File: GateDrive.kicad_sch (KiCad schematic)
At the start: 31 parts, among them Q4 BSS123, U1 UCC21330BQDRQ1, U4 IR2184

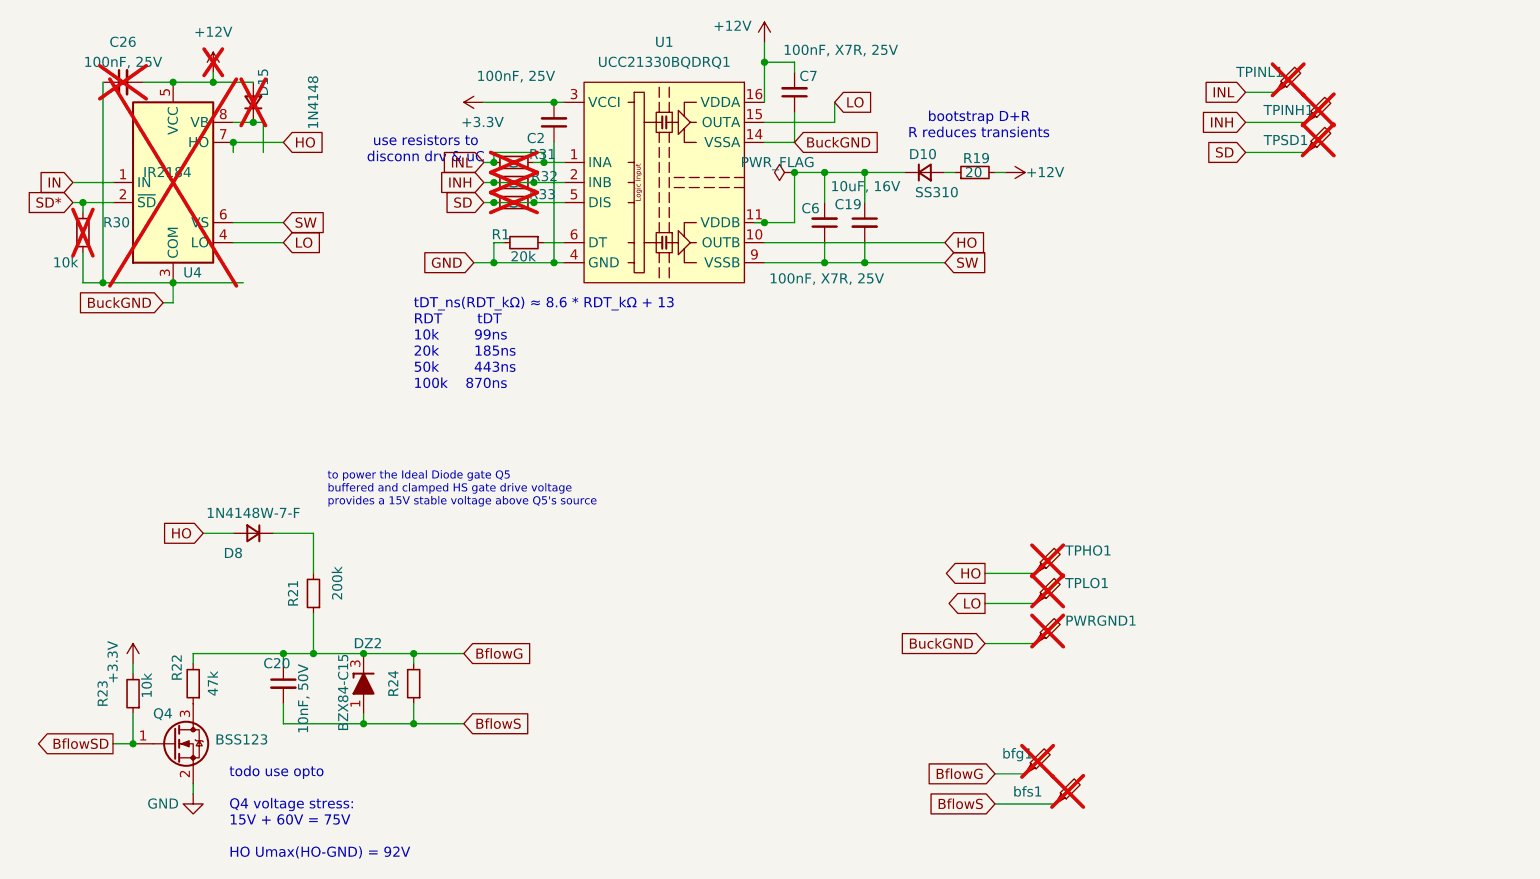
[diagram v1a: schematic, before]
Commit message: First cut, with refactored schematic (PCB now busted, it's a WIP)
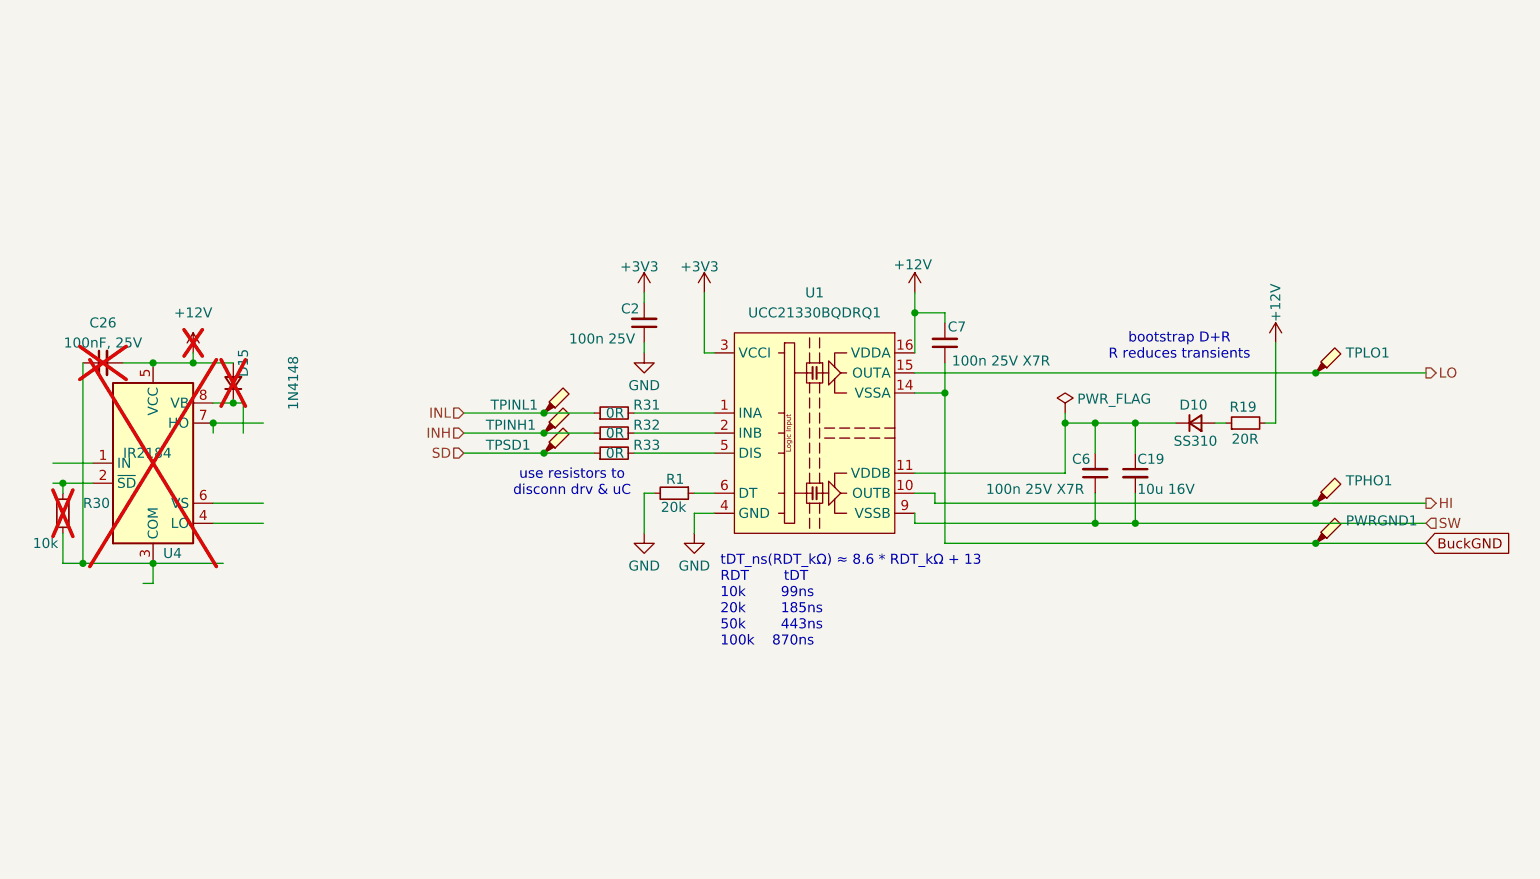
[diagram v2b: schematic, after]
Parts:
- removed C20: 10nF, 50V, Capacitor_SMD:C_0805_2012Metric, symbol Device:C_Small
- removed D8: 1N4148W-7-F, Diode_SMD:D_SOD-123, symbol Device:D_Small
- removed DZ2: BZX84-C15, Package_TO_SOT_SMD:SOT-23, symbol PCM_Diode_Zener_AKL:BZX84-C15
- removed Q4: BSS123, Package_TO_SOT_SMD:SOT-23, symbol Transistor_FET:BSS123
- removed R21: 200k, Resistor_SMD:R_0805_2012Metric, symbol Device:R_Small
- removed R22: 47k, Resistor_SMD:R_0805_2012Metric, symbol Device:R_Small
- removed R23: 10k, Resistor_SMD:R_0805_2012Metric, symbol Device:R_Small
- removed R24: 1M, Resistor_SMD:R_0805_2012Metric, symbol Device:R_Small
- removed bfg1, bfs1: ~, TestPoint:TestPoint_Pad_D1.5mm, symbol Connector:TestPoint_Probe
- C19: value 10uF, 16V -> 10u 16V
- C2: value 100nF, 25V -> 100n 25V
- C6, C7: value 100nF, X7R, 25V -> 100n 25V X7R
- PWRGND1, TPHO1, TPLO1: now fitted; now in the parts list
- R19: value 20 -> 20R
- R31, R32, R33: value 0 -> 0R; footprint Resistor_SMD:R_0402_1005Metric -> Resistor_SMD:R_0603_1608Metric; now fitted; now in the parts list
- TPINH1, TPINL1, TPSD1: now fitted
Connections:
- net BuckGND: no longer C26.1, R30.1, U4.3 (COM)
- net INH: no longer R32.2, U1.2 (INB)
- net INL: no longer R31.2, U1.1 (INA)
- net LO: no longer U4.4 (LO)
- net SD: no longer R33.2, U1.5 (DIS)
- net SW: no longer U4.6 (VS)
- net +3.3V renamed +3V3
- net HO renamed HI
- net HI: no longer U4.7 (HO)
- net IN: no longer names the net of U4.1 (IN)
- net SD*: no longer names the net of R30.2, U4.2 (~{SD})
- new net: R31.2, U1.1 (INA)
- new net: R32.2, U1.2 (INB)
- new net: R33.2, U1.5 (DIS)
- new net: C26.1, R30.1, U4.3 (COM)
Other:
- note removed: "to power the Ideal Diode gate Q5 buffered and clamped HS gate drive voltage provides a 15V stable voltage above Q5's source"
- note removed: "todo use opto Q4 voltage stress: 15V + 60V = 75V HO Umax(HO-GND) = 92V"
- moved on the sheet: C19, C2, C26, C6, C7, D10, D15, R1, R19, R30, U1, U4
